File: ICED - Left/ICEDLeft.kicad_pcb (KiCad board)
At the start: 2 copper layers, 175.4 x 145 mm, 164 parts, among them P1 Conn_ARM_JTAG_SWD_10, P2 DX07S024XJ1R1100, P3 CONN_17, P4 692121130100, P5 RGB Out, Q1 TC1264, U1 MK20DX256VLH7, U2 IS31FL3737-QFLS4-TR, X1 CRYSTAL

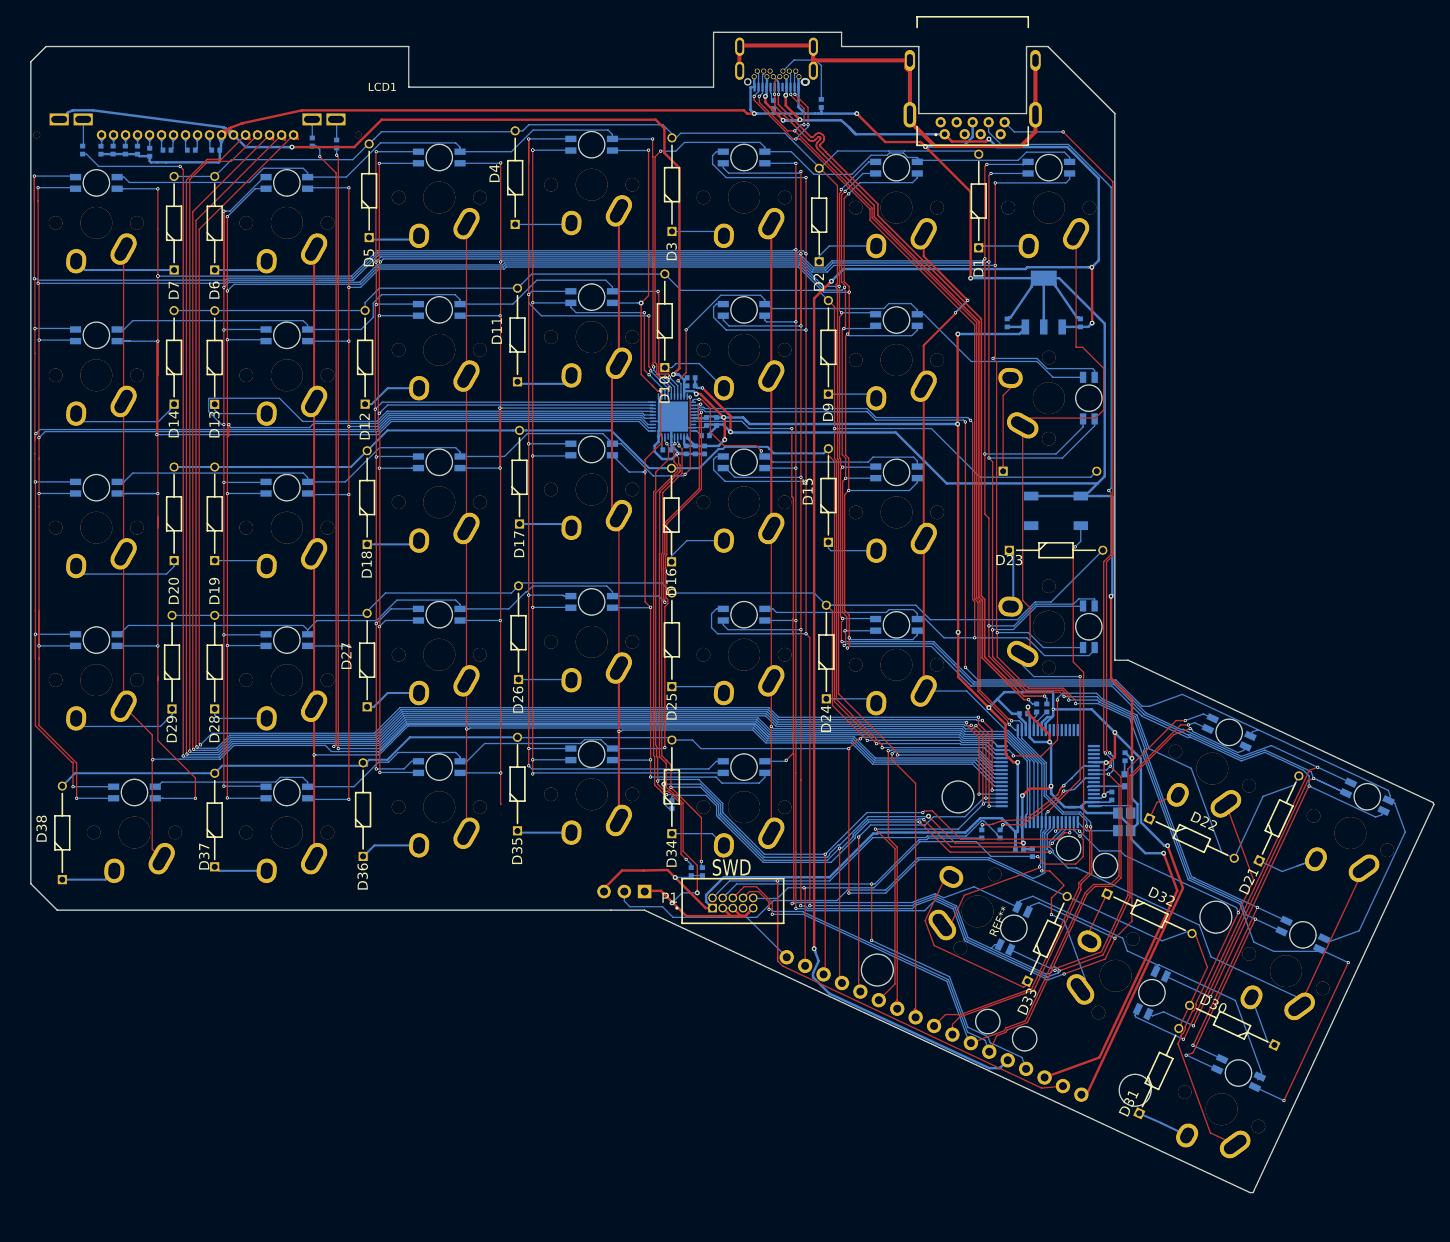
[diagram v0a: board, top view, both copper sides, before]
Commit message: Kailh hotswaps and ground plane
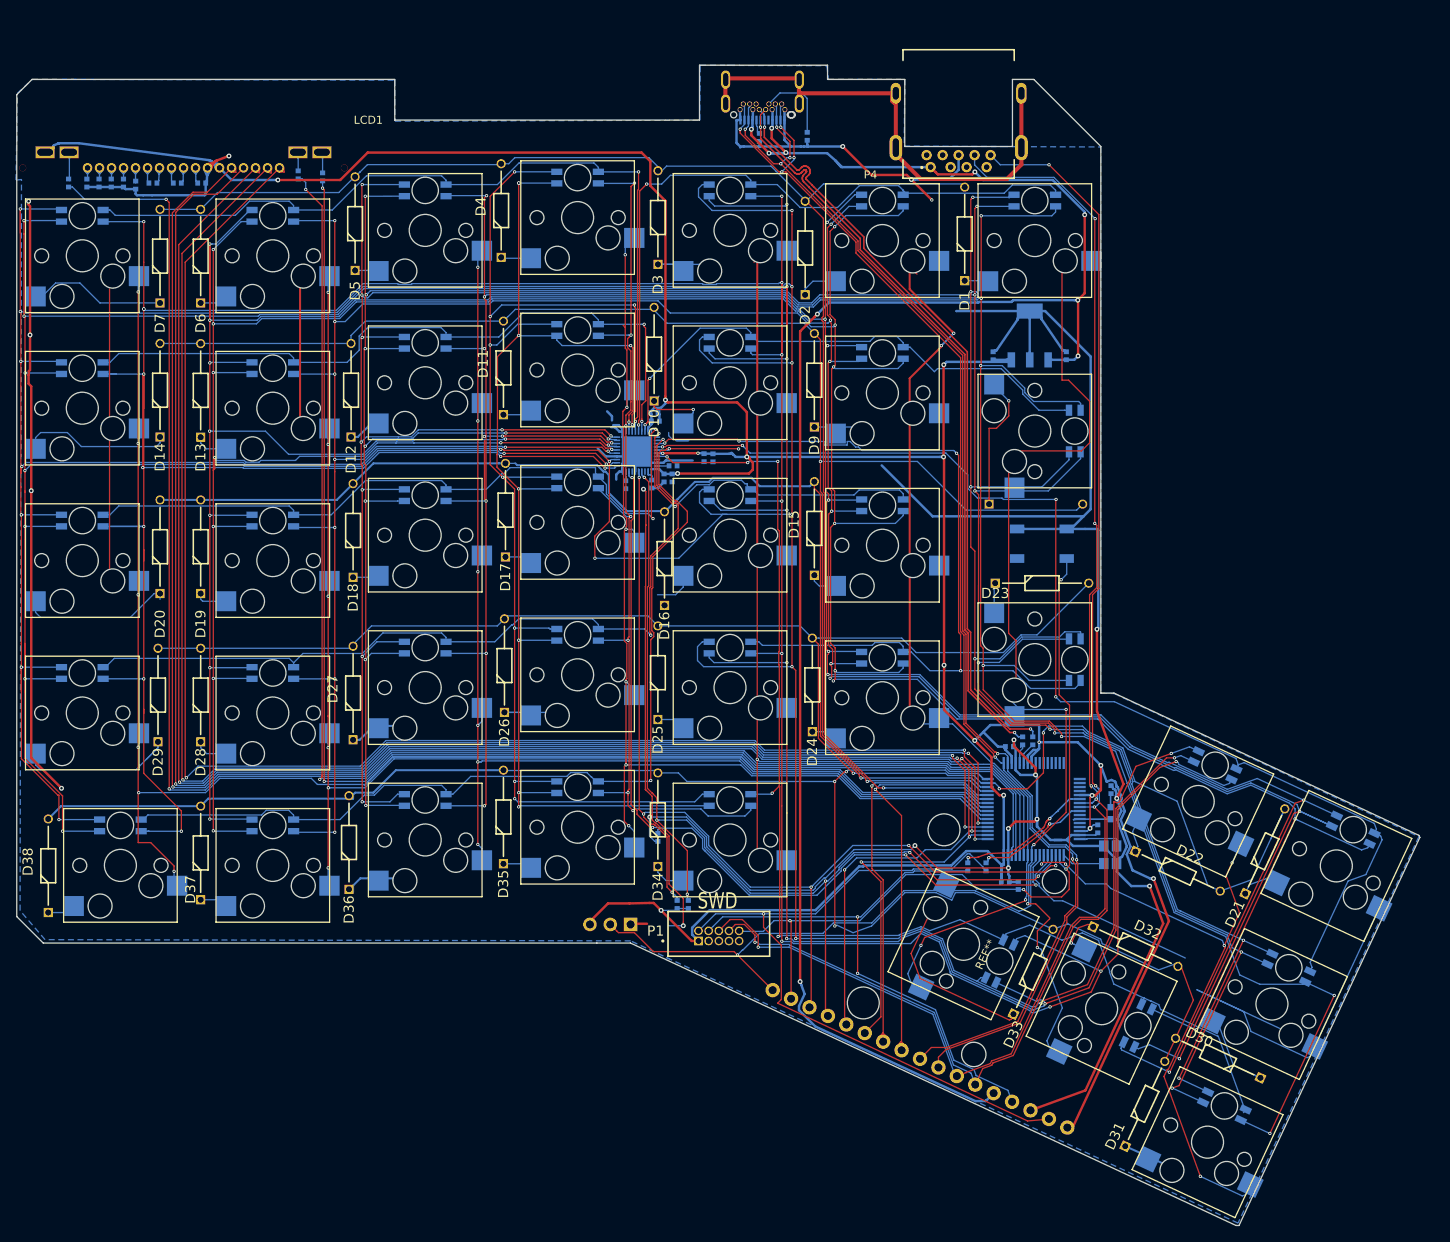
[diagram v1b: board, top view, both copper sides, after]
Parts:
- removed STAB1: Stabilizer_Cherry_MX_2u, prettylib:Stabilizer_Cherry_MX_2u
- S1, S10, S11, S12, S13, S14, S15, S16, S17, S18, S19, S2, S20, S21, S22, S23, S24, S25, S26, S27, S28, S29, S3, S30, S31, S32, S33, S34, S35, S36, S37, S38, S4, S5, S6, S7, S8, S9: footprint prettylib:MXALPS -> prettylib:SW_Hotswap_Kailh
- moved R8 6.75 mm to (85.1, 98.1), turned to 0 degrees
- moved C18 6.38 mm to (88.7, 89.1)
- moved U2 6.27 mm to (86.5, 94.0)
- moved C6 6.27 mm to (88.8, 90.2)
- moved C21 6.05 mm to (88.4, 98.0)
- moved R12 5.53 mm to (91.1, 95.8)
- moved D16 5.51 mm to (90.0, 113.2)
- moved C20 5.34 mm to (90.9, 97.3)
- moved C9 5.25 mm to (89.9, 97.3)
- moved C19 4.56 mm to (96.0, 94.8)
- moved C8 4.53 mm to (94.9, 94.7)
- moved C7 4.47 mm to (144.1, 141.1)
- moved D2 4.47 mm to (107.6, 74.4)
- moved LED10 4.47 mm to (98.2, 80.4)
- moved LED23 4.47 mm to (141.3, 120.0)
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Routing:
- net (no net): track 0.00 -> 192.2 mm, vias 0 -> 2
- net /Col3: track 119.9 -> 58.4 mm
- net /Col4: track 109.5 -> 52.5 mm, vias 3 -> 2
- net VSS: track 596.3 -> 541.9 mm, vias 19 -> 20
- net /mcu/ledmatrix_2/Blue1: track 519.5 -> 549.8 mm, vias 15 -> 18
- net VDD: track 413.0 -> 431.6 mm, vias 16 -> 17
- net /mcu/ledmatrix_2/Blue4: track 161.0 -> 172.5 mm, vias 8 -> 9
- net /Col1: track 64.0 -> 74.8 mm
- net /mcu/ledmatrix_2/Row5A: track 115.2 -> 125.6 mm, vias 2 -> 3
- net /mcu/SWD_DIO: track 100.1 -> 90.5 mm
- net /Col6: track 127.7 -> 136.1 mm, vias 1 -> 6
- net /mcu/ledmatrix_2/Blue2: track 441.8 -> 433.5 mm, vias 15 -> 17
- net /mcu/ledmatrix_2/Row3B: track 35.0 -> 42.9 mm
- net Net-(D29-Pad1): track 13.7 -> 21.6 mm
- net /Col9: track 241.2 -> 247.7 mm, vias 1 -> 6
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- added copper zone on B.Cu, net VSS
